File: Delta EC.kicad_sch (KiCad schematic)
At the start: 42 parts, among them J1 USB_C_Receptacle_USB2.0_16P, J2 Conn_01x08, J3 Conn_01x18, J4 Conn_01x18, U1 STM32G474CBTx, U2 USBLC6-2SC6, U3 TPS7A2033, Y1 8Mhz 12pF

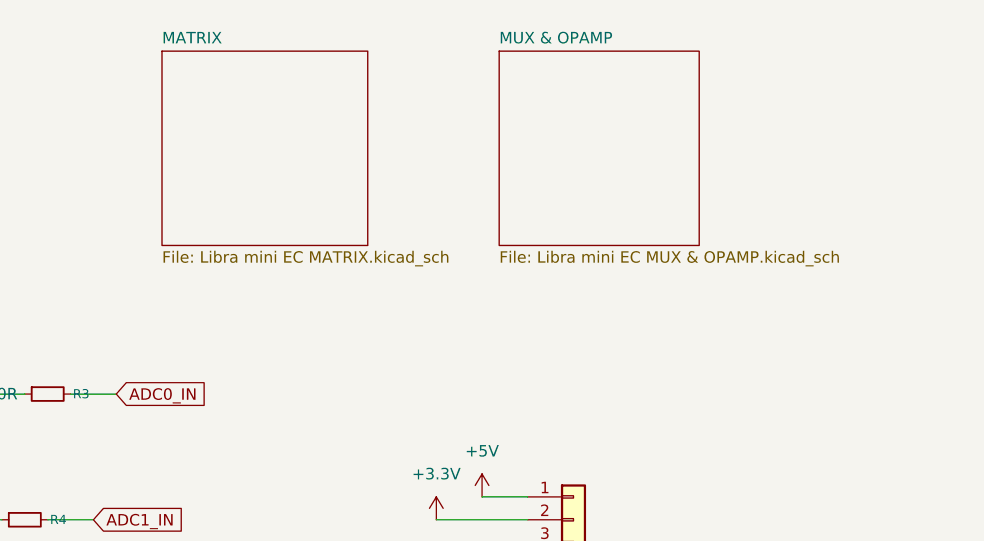
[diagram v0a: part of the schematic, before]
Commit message: 16.04.2026
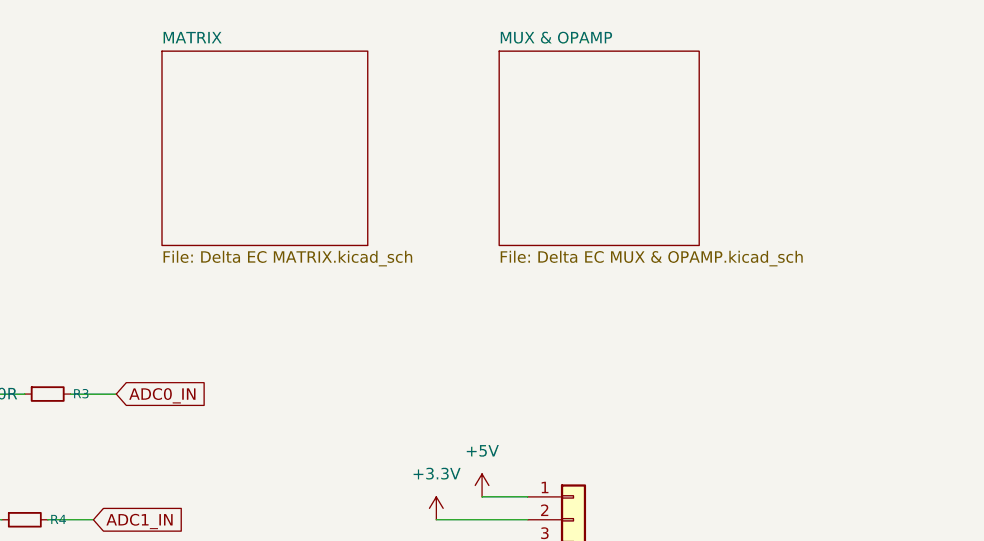
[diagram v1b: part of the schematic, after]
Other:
- sheet MATRIX: file Libra mini EC MATRIX.kicad_sch -> Delta EC MATRIX.kicad_sch
- sheet MUX & OPAMP: file Libra mini EC MUX & OPAMP.kicad_sch -> Delta EC MUX & OPAMP.kicad_sch
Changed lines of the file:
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@@
 			)
 		)
-		(property "Sheetfile" "Libra mini EC MUX & OPAMP.kicad_sch"
+		(property "Sheetfile" "Delta EC MUX & OPAMP.kicad_sch"
 			(at 239.395 38.6846 0)
 			(effects
@@
 		)
 		(instances
-			(project "Libra mini EC"
+			(project "Delta EC"
 				(path "/142d6811-4cb7-4fa7-a144-e9f0e4418635"
 					(page "3")
@@
 			)
 		)
-		(property "Sheetfile" "Libra mini EC MATRIX.kicad_sch"
+		(property "Sheetfile" "Delta EC MATRIX.kicad_sch"
 			(at 201.93 38.6846 0)
 			(effects
@@
 		)
 		(instances
-			(project "Libra mini EC"
+			(project "Delta EC"
 				(path "/142d6811-4cb7-4fa7-a144-e9f0e4418635"
 					(page "2")
